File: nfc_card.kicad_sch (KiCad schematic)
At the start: 3 parts, among them U1 ST25DV04K-JFR6D3

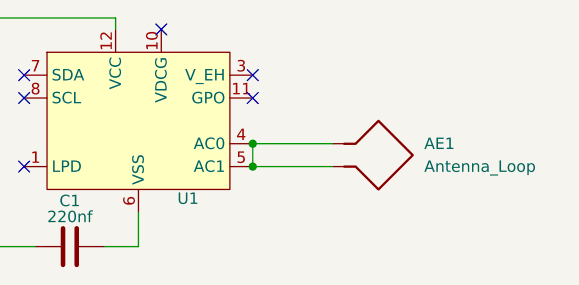
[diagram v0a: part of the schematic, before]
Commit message: a bit of work
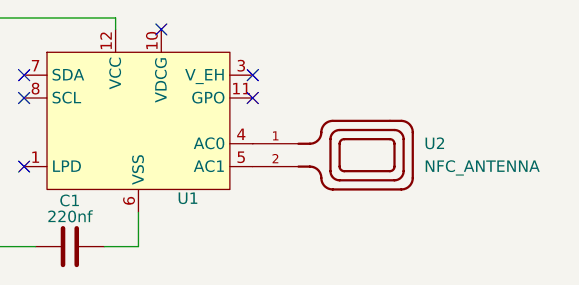
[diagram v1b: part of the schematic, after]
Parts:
- removed AE1: Antenna_Loop, symbol Device:Antenna_Loop
- added U2: NFC_ANTENNA, Library:NFC_ANT, symbol NFC_ANTENNA:NFC_ANTENNA
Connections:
- net at U1.4 (AC0): now also U2.1; no longer U1.5 (AC1)
- new net: U1.5 (AC1), U2.2
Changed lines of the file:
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@@
 	(generator_version "8.0")
 	(paper "A4")
-	(junction
-		(at 124.46 97.79)
-		(diameter 0)
-		(color 0 0 0 0)
-	)
-	(junction
-		(at 124.46 100.33)
-		(diameter 0)
-		(color 0 0 0 0)
-	)
 	(no_connect
 		(at 114.3 85.09)
@@
 	(wire
 		(pts
-			(xy 124.46 100.33) (xy 133.35 100.33)
-		)
-		(stroke
-			(width 0)
-			(type default)
-		)
-	)
-	(wire
-		(pts
 			(xy 107.95 109.22) (xy 111.76 109.22)
 		)
@@
 	(wire
 		(pts
-			(xy 124.46 97.79) (xy 124.46 100.33)
-		)
-		(stroke
-			(width 0)
-			(type default)
-		)
-	)
-	(wire
-		(pts
-			(xy 124.46 97.79) (xy 133.35 97.79)
-		)
-		(stroke
-			(width 0)
-			(type default)
-		)
-	)
-	(wire
-		(pts
 			(xy 109.22 83.82) (xy 109.22 85.09)
 		)
@@
 			(width 0)
 			(type default)
+		)
+	)
+	(symbol
+		(lib_id "NFC_ANTENNA:NFC_ANTENNA")
+		(at 137.16 102.87 0)
+		(unit 1)
+		(exclude_from_sim no)
+		(in_bom yes)
+		(on_board yes)
+		(dnp no)
+		(fields_autoplaced yes)
+		(property "Reference" "U2"
+			(at 143.51 97.7899 0)
+			(effects
+				(font
+					(size 1.27 1.27)
+				)
+				(justify left)
+			)
+		)
+		(property "Value" "NFC_ANTENNA"
+			(at 143.51 100.3299 0)
+			(effects
+				(font
+					(size 1.27 1.27)
+				)
+				(justify left)
+			)
+		)
+		(property "Footprint" "Library:NFC_ANT"
+			(at 137.16 102.87 0)
+			(effects
+				(font
+					(size 1.27 1.27)
+				)
+				(justify bottom)
+				(hide yes)
+			)
+		)
+		(property "Datasheet" ""
+			(at 137.16 102.87 0)
+			(effects
+				(font
+					(size 1.27 1.27)
+				)
+				(hide yes)
+			)
+		)
+		(property "Description" ""
+			(at 137.16 102.87 0)
+			(effects
+				(font
+					(size 1.27 1.27)
+				)
+				(hide yes)
+			)
+		)
+		(property "MF" "DComponents"
+			(at 137.16 102.87 0)
+			(effects
+				(font
+					(size 1.27 1.27)
+				)
+				(justify bottom)
+				(hide yes)
+			)
+		)
+		(property "Description_1" "\nNFC Flex PCB Antenna nRF52832/84\n"
+			(at 137.16 102.87 0)
+			(effects
+				(font
+					(size 1.27 1.27)
+				)
+				(justify bottom)
+				(hide yes)
+			)
+		)
+		(property "Package" "None"
+			(at 137.16 102.87 0)
+			(effects
+				(font
+					(size 1.27 1.27)
+				)
+				(justify bottom)
+				(hide yes)
+			)
+		)
+		(property "Price" "None"
+			(at 137.16 102.87 0)
+			(effects
+				(font
+					(size 1.27 1.27)
+				)
+				(justify bottom)
+				(hide yes)
+			)
+		)
+		(property "SnapEDA_Link" "https://www.snapeda.com/parts/NFC%20Antenna/RND/view-part/?ref=snap"
+			(at 137.16 102.87 0)
+			(effects
+				(font
+					(size 1.27 1.27)
+				)
+				(justify bottom)
+				(hide yes)
+			)
+		)
+		(property "MP" "NFC Antenna"
+			(at 137.16 102.87 0)
+			(effects
+				(font
+					(size 1.27 1.27)
+				)
+				(justify bottom)
+				(hide yes)
+			)
+		)
+		(property "Availability" "Not in stock"
+			(at 137.16 102.87 0)
+			(effects
+				(font
+					(size 1.27 1.27)
+				)
+				(justify bottom)
+				(hide yes)
+			)
+		)
+		(property "Check_prices" "https://www.snapeda.com/parts/NFC%20Antenna/RND/view-part/?ref=eda"
+			(at 137.16 102.87 0)
+			(effects
+				(font
+					(size 1.27 1.27)
+				)
+				(justify bottom)
+				(hide yes)
+			)
+		)
+		(pin "1"
+		)
+		(pin "2"
+		)
+		(instances
+			(project ""
+				(path "/1b8f39ab-cd0d-4acb-ac11-96af87f86161"
+					(reference "U2")
+					(unit 1)
+				)
+			)
 		)
 	)
@@
 					(unit 1)
 				)
-			)
-		)
-	)
-	(symbol
-		(lib_id "Device:Antenna_Loop")
-		(at 138.43 97.79 270)
-		(unit 1)
-		(exclude_from_sim no)
-		(in_bom yes)
-		(on_board yes)
-		(dnp no)
-		(fields_autoplaced yes)
-		(property "Reference" "AE1"
-			(at 143.51 97.7899 90)
-			(effects
-				(font
-					(size 1.27 1.27)
-				)
-				(justify left)
-			)
-		)
-		(property "Value" "Antenna_Loop"
-			(at 143.51 100.3299 90)
-			(effects
-				(font
-					(size 1.27 1.27)
-				)
-				(justify left)
-			)
-		)
-		(property "Footprint" ""
-			(at 138.43 97.79 0)
-			(effects
-				(font
-					(size 1.27 1.27)
-				)
-				(hide yes)
-			)
-		)
-		(property "Datasheet" "~"
-			(at 138.43 97.79 0)
-			(effects
-				(font
-					(size 1.27 1.27)
-				)
-				(hide yes)
-			)
-		)
-		(property "Description" "Loop antenna"
-			(at 138.43 97.79 0)
-			(effects
-				(font
-					(size 1.27 1.27)
-				)
-				(hide yes)
-			)
-		)
-		(pin "2"
-		)
-		(pin "1"
-		)
-		(instances
-			(project ""
-				(path "/1b8f39ab-cd0d-4acb-ac11-96af87f86161"
-					(reference "AE1")
-					(unit 1)
-				)

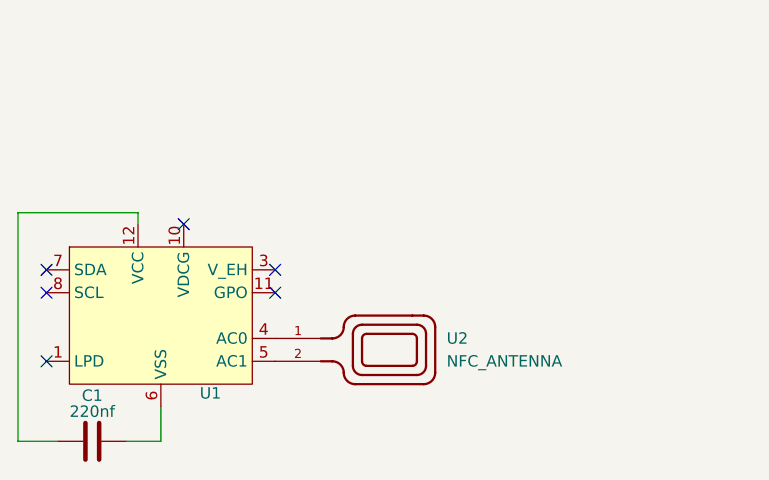
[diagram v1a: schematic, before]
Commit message: graphics!
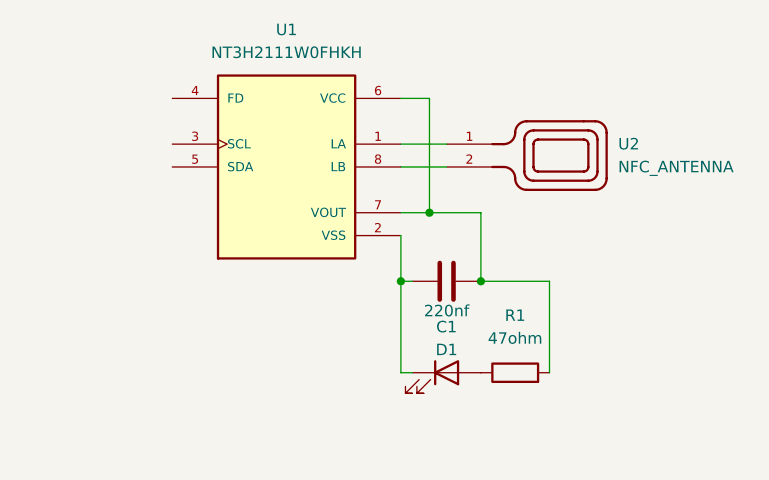
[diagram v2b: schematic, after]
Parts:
- removed U1: ST25DV04K-JFR6D3, Package_DFN_QFN:ST_UFDFPN-12-1EP_3x3mm_P0.5mm_EP1.4x2.55mm, symbol RF_NFC:ST25DV04K-JFR6D3
- added D1: LED, symbol Device:LED
- added R1: 47ohm, symbol Device:R
- added U1: NT3H2111W0FHKH, NT3H2111W0FHKH:QFN8P50_160X160X50L40X20N, symbol NT3H2111W0FHKH:NT3H2111W0FHKH
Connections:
- net at U2.1: now also U1.1 (LA)
- net at U2.2: now also U1.8 (LB)
- net at C1.1: now also R1.2, U1.6 (VCC), U1.7 (VOUT)
- net at C1.2: now also D1.1 (K), U1.2 (VSS)
- new net: D1.2 (A), R1.1
- no-connect marks 6 -> 0
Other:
- moved on the sheet: U2
